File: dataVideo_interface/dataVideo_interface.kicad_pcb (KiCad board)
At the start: 2 copper layers, 2 parts, among them J1 Conn_in, J2 Conn_out

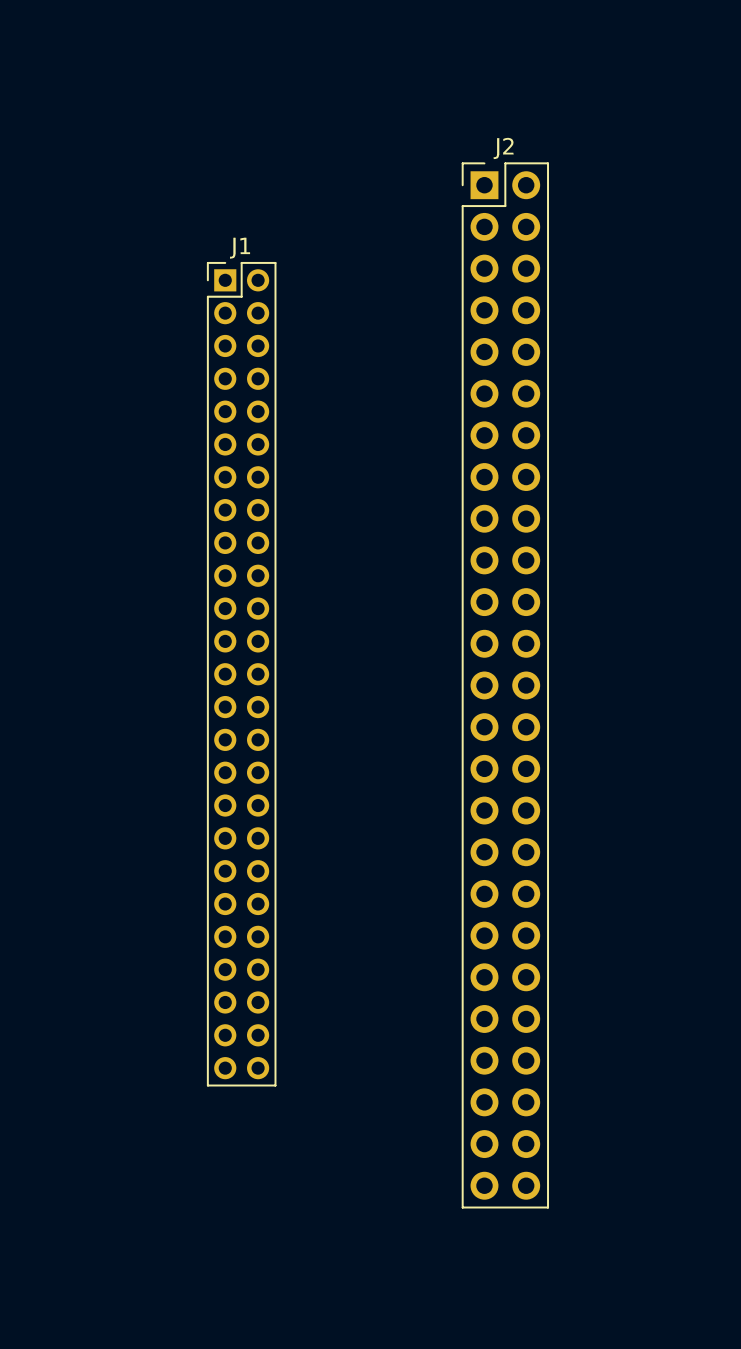
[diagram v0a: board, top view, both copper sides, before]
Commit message: first revision and production files
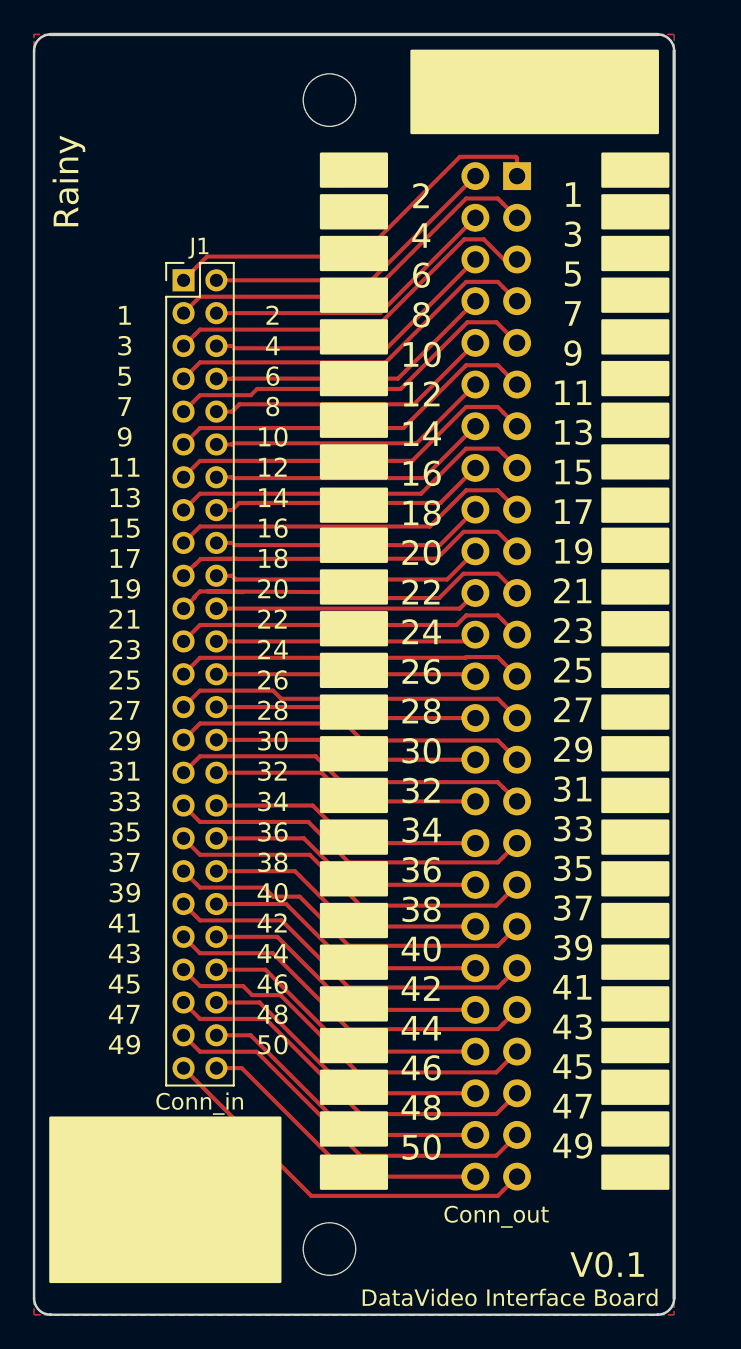
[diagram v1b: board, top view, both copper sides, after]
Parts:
- added REF**: MountingHole_3.2mm_M3_ISO14580, Mounting_Holes:MountingHole_3.2mm_M3_ISO14580, F.Cu at (127.0, 153.0)
- added REF**: MountingHole_3.2mm_M3_ISO14580, Mounting_Holes:MountingHole_3.2mm_M3_ISO14580, F.Cu at (127.0, 83.0)
- J2: moved to B.Cu
- moved J1 2.54 mm to (118.1, 94.0)
- moved J2 2.06 mm to (138.4, 87.6), turned to 180 degrees
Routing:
- net 1: track 0.00 -> 24.6 mm
- net 21: track 0.00 -> 24.2 mm
- net 49: track 0.00 -> 24.0 mm
- net 47: track 0.00 -> 23.9 mm
- net 3: track 0.00 -> 23.7 mm
- net 19: track 0.00 -> 23.7 mm
- net 45: track 0.00 -> 23.7 mm
- net 5: track 0.00 -> 23.6 mm
- net 43: track 0.00 -> 23.4 mm
- net 7: track 0.00 -> 23.3 mm
- net 41: track 0.00 -> 23.1 mm
- net 9: track 0.00 -> 23.1 mm
- net 39: track 0.00 -> 22.9 mm
- net 11: track 0.00 -> 22.8 mm
- net 37: track 0.00 -> 22.7 mm
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- added copper zone on B.Cu, net (none)
- added copper zone on F.Cu, net (none)
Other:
- board outline added: 39 x 78 mm
- board text added: "1 3 5 7 9 11 13 15 17 19 21 23 25 27 29 31 33 35 37 39 41 43 45 47 49"
- board text added: "2 4 6 8 10 12 14 16 18 20 22 24 26 28 30 32 34 36 38 40 42 44 46 48 50"
- board text added: "DataVideo Interface Board"
- board text added: "Rainy"
- board text added: "V0.1"
